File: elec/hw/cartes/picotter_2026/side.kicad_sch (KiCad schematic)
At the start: 18 parts, among them J3 5264-3P, J4 22053051, J5 22053051, J6 22272041, J7 22272051, U2 VCNL4040M3OE

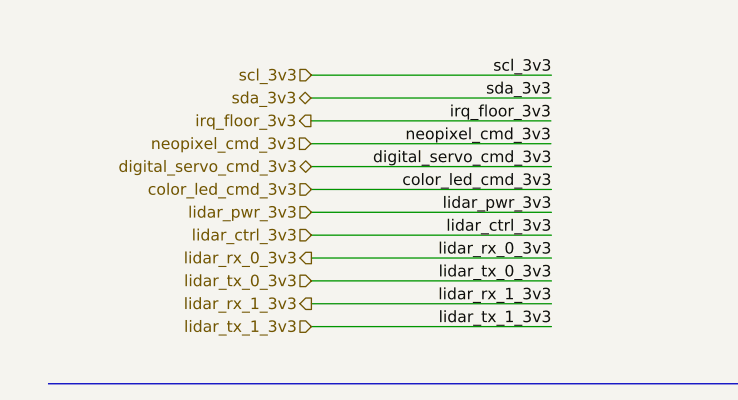
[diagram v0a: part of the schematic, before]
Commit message: picotter: final layout
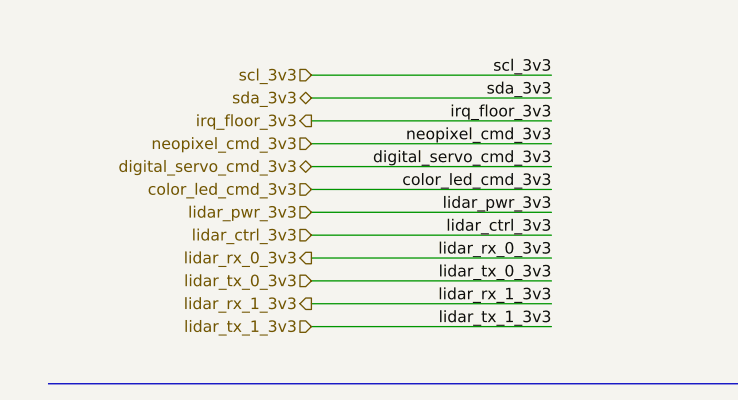
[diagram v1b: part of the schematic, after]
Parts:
- U2: footprint cocotter_ic:VISHAY_VCNL4040_4X2X1.1 -> VCNL4040M3OE:VISHAY_VCNL4040_4X2X1.1
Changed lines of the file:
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@@
-	(wire
-		(pts
-			(xy 41.8506 21.59) (xy 68.5206 21.59)
-		)
-		(stroke
-			(width 0)
-			(type default)
-		)
-	)
 	(wire
 		(pts
@@
 	(wire
 		(pts
-			(xy 41.8506 24.13) (xy 68.5206 24.13)
-		)
-		(stroke
-			(width 0)
-			(type default)
-		)
-	)
-	(wire
-		(pts
 			(xy 19.05 95.25) (xy 41.91 95.25)
 		)
@@
 	(wire
 		(pts
-			(xy 41.8506 26.67) (xy 68.5206 26.67)
-		)
-		(stroke
-			(width 0)
-			(type default)
-		)
-	)
-	(wire
-		(pts
 			(xy 104.14 72.39) (xy 104.14 74.93)
 		)
@@
 	(wire
 		(pts
+			(xy 41.91 24.13) (xy 68.58 24.13)
+		)
+		(stroke
+			(width 0)
+			(type default)
+		)
+	)
+	(wire
+		(pts
 			(xy 237.49 101.6) (xy 240.03 101.6)
 		)
@@
 	(wire
 		(pts
+			(xy 41.91 21.59) (xy 68.58 21.59)
+		)
+		(stroke
+			(width 0)
+			(type default)
+		)
+	)
+	(wire
+		(pts
 			(xy 76.2 69.85) (xy 76.2 72.39)
 		)
@@
 		(pts
 			(xy 53.34 138.43) (xy 53.34 165.1)
+		)
+		(stroke
+			(width 0)
+			(type default)
+		)
+	)
+	(wire
+		(pts
+			(xy 41.91 26.67) (xy 68.58 26.67)
 		)
 		(stroke
@@
 	)
 	(label "irq_floor_3v3"
-		(at 68.5206 24.13 180)
+		(at 68.58 24.13 180)
 		(effects
 			(font
@@
 	)
 	(label "neopixel_cmd_3v3"
-		(at 68.5206 26.67 180)
+		(at 68.58 26.67 180)
 		(effects
 			(font
@@
 	)
 	(label "sda_3v3"
-		(at 68.5206 21.59 180)
+		(at 68.58 21.59 180)
 		(effects
 			(font
@@
 	(hierarchical_label "irq_floor_3v3"
 		(shape output)
-		(at 41.8506 24.13 180)
+		(at 41.91 24.13 180)
 		(effects
 			(font
@@
 	(hierarchical_label "neopixel_cmd_3v3"
 		(shape input)
-		(at 41.8506 26.67 180)
+		(at 41.91 26.67 180)
 		(effects
 			(font
@@
 	(hierarchical_label "sda_3v3"
 		(shape bidirectional)
-		(at 41.8506 21.59 180)
+		(at 41.91 21.59 180)
 		(effects
 			(font
@@
 			)
 		)
-		(property "Footprint" "cocotter_ic:VISHAY_VCNL4040_4X2X1.1"
+		(property "Footprint" "VCNL4040M3OE:VISHAY_VCNL4040_4X2X1.1"
 			(at 78.74 95.25 0)
 			(effects
